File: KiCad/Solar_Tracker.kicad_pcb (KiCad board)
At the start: 2 copper layers, 160 x 100 mm, 119 parts, among them J1 +48V, J10 AZJMP, J11 ELJMP, J12 AZ, J13 CONN_01X03, J2 HOLE, J3 HOLE, J4 EL, J5 HOLE, J6 HOLE, J7 CONN_01X05, J8 GPIO, J9 GPIO, Q1 BUK9M42-60E, Q2 BUK9M42-60E, Q3 BUK9M42-60E, Q4 BUK9M42-60E, Q5 BUK9M42-60E, Q6 BUK9M42-60E, Q7 BUK9M42-60E, Q8 BUK9M42-60E, U1 MER1S4805SC, U10 TLP291, U11 75LBC182, U12 A4927, U13 PCA9685, U2 A4927, U3 Nano, U4 A4927, U5 A4927, U6 MER1S4805SC, U7 TLP291, U8 TLP291, U9 TLP291

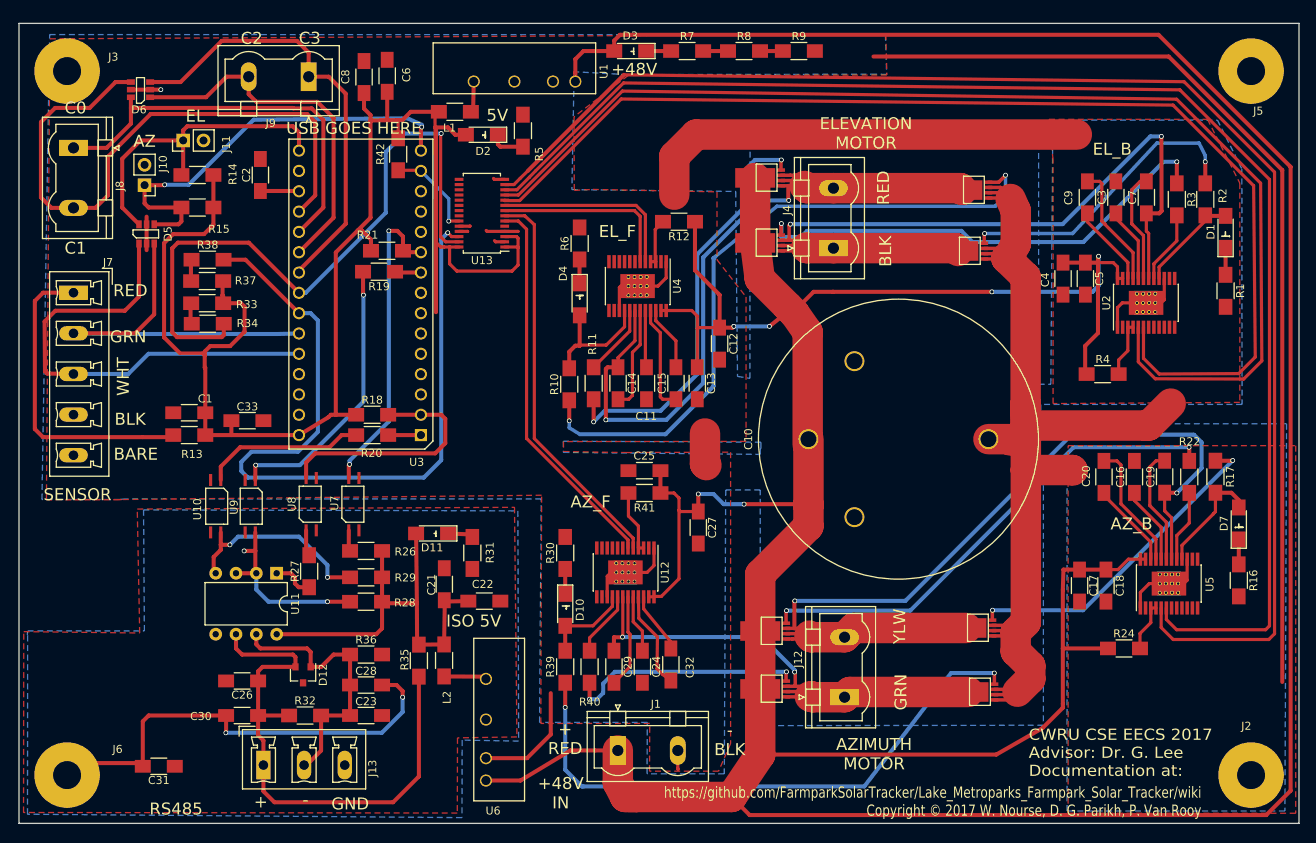
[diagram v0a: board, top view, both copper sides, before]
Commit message: Updated documentation
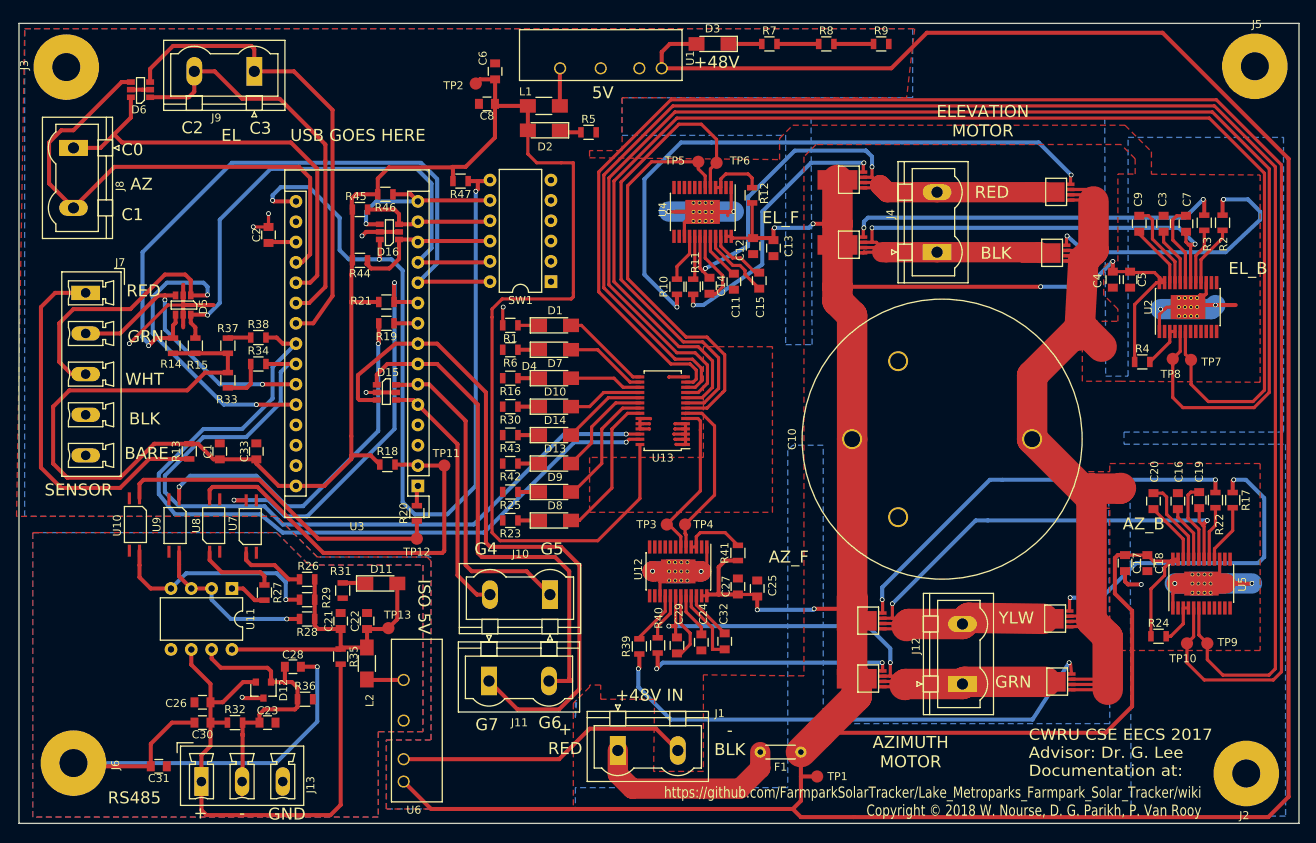
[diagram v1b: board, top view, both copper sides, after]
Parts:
- added D13: STAT2, LEDs:LED_1206_HandSoldering, F.Cu at (79.0, 67.1)
- added D14: STAT1, LEDs:LED_1206_HandSoldering, F.Cu at (79.0, 63.5)
- added D15: TVS_x4, SOLAR:tvs_quad, F.Cu at (57.9, 58.2)
- added D16: TVS_x4, SOLAR:tvs_quad, F.Cu at (58.3, 38.1)
- added D8: STAT4, LEDs:LED_1206_HandSoldering, F.Cu at (79.0, 74.2)
- added D9: STAT3, LEDs:LED_1206_HandSoldering, F.Cu at (79.0, 70.6)
- added F1: Fuse, Resistors_THT:R_Axial_DIN0204_L3.6mm_D1.6mm_P5.08mm_Horizontal, F.Cu at (109.7, 103.1)
- added R23: 150, Resistors_SMD:R_0805, F.Cu at (73.4, 74.2)
- added R25: 150, Resistors_SMD:R_0805, F.Cu at (73.4, 70.6)
- added R43: 150, Resistors_SMD:R_0805, F.Cu at (73.4, 63.5)
- added R44: 1K, Resistors_SMD:R_0805, F.Cu at (54.6, 41.7)
- added R45: 1K, Resistors_SMD:R_0805, F.Cu at (54.6, 35.3)
- added R46: 1K, Resistors_SMD:R_0805, F.Cu at (57.8, 33.4)
- added R47: 1K, Resistors_SMD:R_0805, F.Cu at (67.2, 31.8)
- added SW1: DIPSWITCH, Housings_DIP:DIP-12_W7.62mm, F.Cu at (78.5, 44.3)
- added TP1: +48V, SOLAR:test_pad, F.Cu at (111.8, 106.2)
- added TP10: AZBH, SOLAR:test_pad, F.Cu at (158.0, 89.5)
- added TP11: RX, SOLAR:test_pad, F.Cu at (65.2, 67.3)
- added TP12: TX, SOLAR:test_pad, F.Cu at (61.7, 76.5)
- added TP13: +5V_ISO, SOLAR:test_pad, F.Cu at (58.2, 87.6)
- added TP2: +5V, SOLAR:test_pad, F.Cu at (69.1, 19.6)
- added TP3: AZFL, SOLAR:test_pad, F.Cu at (93.0, 74.7)
- added TP4: AZFH, SOLAR:test_pad, F.Cu at (95.2, 74.7)
- added TP5: ELFL, SOLAR:test_pad, F.Cu at (96.9, 29.3)
- added TP6: ELFH, SOLAR:test_pad, F.Cu at (99.2, 29.5)
- added TP7: ELBL, SOLAR:test_pad, F.Cu at (158.5, 54.1)
- added TP8: ELBH, SOLAR:test_pad, F.Cu at (156.2, 54.0)
- added TP9: AZBL, SOLAR:test_pad, F.Cu at (160.5, 89.5)
- C1, C11, C12, C13, C14, C15, C16, C17, C18, C19, C2, C20, C21, C22, C23, C24, C25, C26, C27, C28, C29, C3, C30, C31, C32, C33, C4, C5, C6, C7, C8, C9: footprint Capacitors_SMD:C_1206_HandSoldering -> Capacitors_SMD:C_0805
- C10: footprint SOLAR_TRACKER:vnd_cap -> SOLAR:vnd_cap
- D5, D6: footprint SOLAR_TRACKER:tvs_quad -> SOLAR:tvs_quad
- J10: value AZJMP -> GPIO; footprint Pin_Headers:Pin_Header_Straight_1x02_Pitch2.54mm -> Connectors_Phoenix:PhoenixContact_GMSTBVA-G_02x7.50mm_Vertical
- J11: value ELJMP -> GPIO; footprint Pin_Headers:Pin_Header_Straight_1x02_Pitch2.54mm -> Connectors_Phoenix:PhoenixContact_GMSTBVA-G_02x7.50mm_Vertical
- J2, J3, J5, J6: footprint SOLAR_TRACKER:M3 -> SOLAR:M3
- Q1, Q2, Q3, Q4, Q5, Q6, Q7, Q8: footprint SOLAR_TRACKER:nFET -> SOLAR:nFET
- R1, R10, R11, R12, R13, R14, R15, R16, R17, R18, R19, R2, R20, R21, R22, R24, R26, R27, R28, R29, R3, R30, R31, R32, R33, R34, R35, R36, R37, R38, R39, R4, R40, R41, R5, R6, R7, R8, R9: footprint Resistors_SMD:R_1206_HandSoldering -> Resistors_SMD:R_0805
- R42: value 1K -> 150; footprint Resistors_SMD:R_1206_HandSoldering -> Resistors_SMD:R_0805
- U1, U6: footprint SOLAR_TRACKER:5v_iso -> SOLAR:5v_iso
- U10, U7, U8, U9: footprint SOLAR_TRACKER:opto -> SOLAR:opto
- U3: footprint SOLAR_TRACKER:nano -> Modules:Arduino_Nano
- moved R16 94.5 mm to (73.4, 56.4), turned to 180 degrees
- moved R1 89.5 mm to (73.4, 49.8), turned to 180 degrees
- moved D7 87.4 mm to (79.0, 56.4), turned to 0 degrees
- moved D1 84.6 mm to (79.0, 49.8), turned to 0 degrees
- moved J11 77.6 mm to (70.7, 94.2), turned to 0 degrees
- moved J10 72.0 mm to (78.4, 83.4)
- moved R42 41.1 mm to (73.4, 67.1), turned to 180 degrees
- moved U13 33.5 mm to (92.5, 60.5)
- moved D10 25.4 mm to (79.0, 59.9), turned to 0 degrees
- moved R14 21.6 mm to (31.2, 52.3), turned to 270 degrees
- moved C25 20.4 mm to (104.3, 82.7), turned to 90 degrees
- moved R30 19.5 mm to (73.4, 59.9), turned to 180 degrees
- moved C13 19.4 mm to (106.3, 40.1)
- moved R10 18.2 mm to (94.2, 45.0)
- moved R11 17.3 mm to (96.3, 45.0)
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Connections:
- net C0 renamed G0
- net C1 renamed G1
- net C2 renamed G2
- net C3 renamed G3
- D5 pad 4: AZRTE -> SEL0
- D5 pad 6: ELRTE -> SEL1
- J1 pad 1: +48V -> Net-(F1-Pad2)
- J10 pad 1: AZRTE -> G5
- J10 pad 2: GND -> G4
- J11 pad 1: ELRTE -> G7
- J11 pad 2: GND -> G6
- R10 pad 2: Net-(D4-Pad2) -> Net-(R10-Pad2)
- R14 pad 1: ELRTE -> SEL0
- R15 pad 1: AZRTE -> SEL1
- R17 pad 2: Net-(D7-Pad2) -> Net-(R17-Pad2)
- R2 pad 2: Net-(D1-Pad2) -> Net-(R2-Pad2)
- R39 pad 2: Net-(D10-Pad2) -> Net-(R39-Pad2)
- R42 pad 1: +5V -> Net-(D13-Pad1)
- R42 pad 2: Net-(R42-Pad2) -> GND
- U12 pad 16: Net-(D10-Pad2) -> Net-(R39-Pad2)
- U13 pad 1: +5V -> GND
- U13 pad 15: Net-(U13-Pad15) -> Net-(D1-Pad2)
- U13 pad 16: Net-(U13-Pad16) -> Net-(D4-Pad2)
- U13 pad 17: Net-(U13-Pad17) -> Net-(D7-Pad2)
- U13 pad 18: Net-(U13-Pad18) -> Net-(D10-Pad2)
- U13 pad 23: Net-(R42-Pad2) -> GND
- U13 pad 26: Net-(R38-Pad2) -> Net-(R34-Pad2)
- U13 pad 27: Net-(R34-Pad2) -> Net-(R38-Pad2)
- U13 pad 3: +5V -> GND
- U13 pad 5: +5V -> GND
- U2 pad 16: Net-(D1-Pad2) -> Net-(R2-Pad2)
- U3 pad 11: Net-(U3-Pad11) -> SEL0
- U3 pad 12: Net-(U3-Pad12) -> SEL1
- U3 pad 13: Net-(U3-Pad13) -> SEL2
- U3 pad 14: Net-(R42-Pad2) -> SEL3
- U3 pad 15: AZRTE -> SEL4
- U3 pad 16: ELRTE -> SEL5
- U3 pad 23: Net-(R34-Pad2) -> Net-(R38-Pad2)
- U3 pad 24: Net-(R38-Pad2) -> Net-(R34-Pad2)
- U3 pad 5: Net-(U3-Pad5) -> G4
- U3 pad 6: Net-(U3-Pad6) -> G5
- U3 pad 7: Net-(U3-Pad7) -> G6
- U3 pad 8: Net-(U3-Pad8) -> G7
- U4 pad 16: Net-(D4-Pad2) -> Net-(R10-Pad2)
- U5 pad 16: Net-(D7-Pad2) -> Net-(R17-Pad2)
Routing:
- net SEL5: track 0.00 -> 110.7 mm, vias 0 -> 3
- net G7: track 0.00 -> 86.3 mm
- net SEL0: track 0.00 -> 83.8 mm, vias 0 -> 1
- net SEL1: track 0.00 -> 67.4 mm, vias 0 -> 1
- net G6: track 0.00 -> 64.1 mm
- net AZRTE: track 53.9 -> 0.00 mm, vias 2 -> 0
- net G5: track 0.00 -> 40.7 mm
- net ELRTE: track 40.6 -> 0.00 mm
- net +48V: track 601.7 -> 563.2 mm
- net ELFH: track 23.9 -> 59.2 mm
- net +5V: track 223.5 -> 258.0 mm
- net GND: track 378.5 -> 346.1 mm, vias 1 -> 15
- net G4: track 0.00 -> 31.4 mm
- net AZ_B: track 108.3 -> 77.7 mm
- net ELFL: track 22.9 -> 51.6 mm
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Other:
- board text added: "G4"
- board text added: "G5"
- board text added: "G6"
- board text added: "G7"
- board text added: "https://github.com/FarmparkSolarTracker/Lake_Metroparks_Farmpark_Solar_Tracker/wiki Copyright © 2018 W. Nourse, D. G. Parikh, P. Van Rooy"
- board text removed: "https://github.com/FarmparkSolarTracker/Lake_Metroparks_Farmpark_Solar_Tracker/wiki Copyright © 2017 W. Nourse, D. G. Parikh, P. Van Rooy"
